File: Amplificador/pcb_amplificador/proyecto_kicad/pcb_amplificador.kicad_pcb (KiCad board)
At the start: 2 copper layers, 149.9 x 88.9 mm, 140 parts, among them CON1 SJ-3523-SMT-TR, J1 Screw_Terminal_01x02, J2 Screw_Terminal_01x02, J3 Screw_Terminal_01x02, J4 Screw_Terminal_01x02, J5 Conn_01x03_Male, J6 Screw_Terminal_01x02, J7 Screw_Terminal_01x02, K1 FINDER-40.11-2016, M1 FDS9934C, M2 FDS9934C, Q1 BC860, Q10 BD139, Q11 BD140, Q12 BD139, Q13 2SA1943-O_Q_, Q14 2SC5200-O_Q, Q15 2SA1943-O_Q_, Q16 2SC5200-O_Q, Q17 2SAR514P5, Q18 BC860, Q19 BC860, Q2 BC860, Q20 2SAR514P5, Q21 2SCR514P5, Q22 2SCR514P5, Q23 2SCR514P5, Q24 2SAR514P5, Q25 2SCR514P5, Q26 BC817, Q27 BC817, Q28 BC807, Q29 BS170, Q3 BC850, Q4 BC850, Q5 BC860, Q6 BC860, Q7 BC850, Q8 2SCR514P5, Q9 2SCR514P5

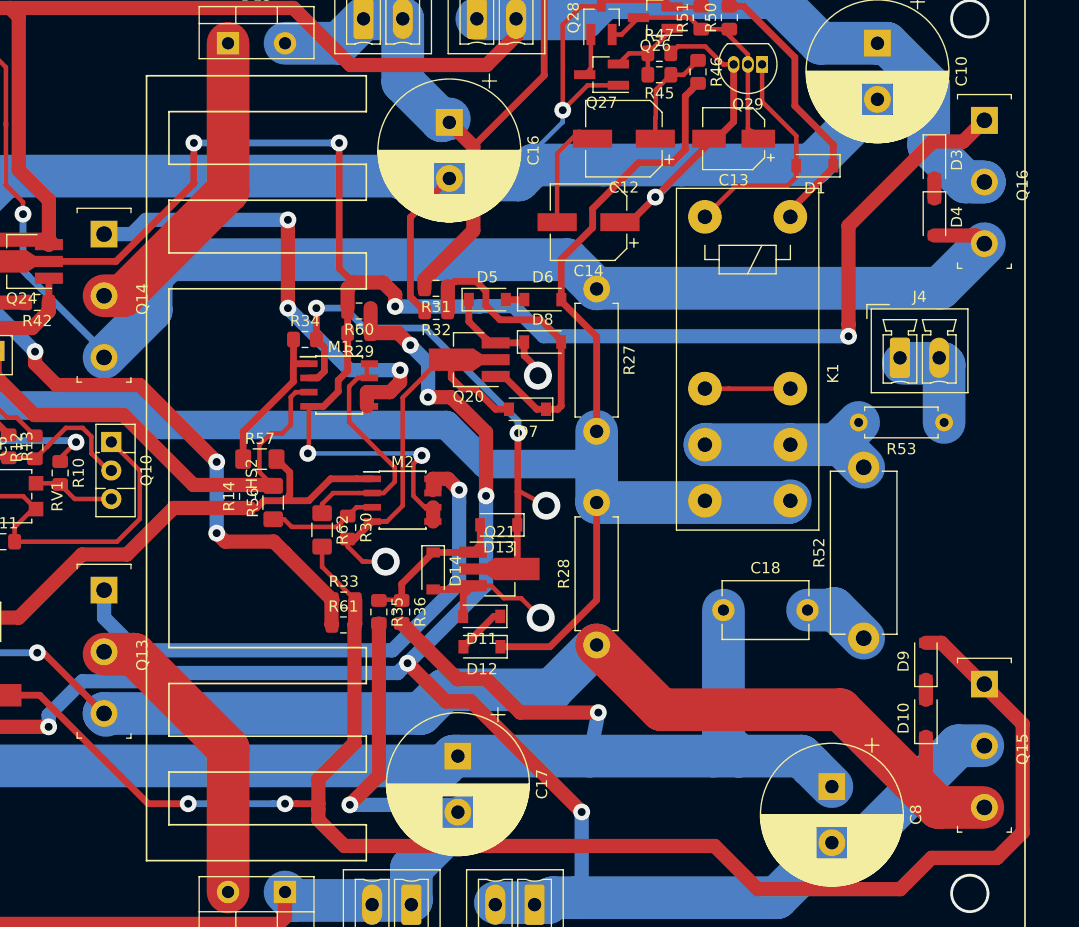
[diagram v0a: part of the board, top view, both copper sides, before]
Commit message: Agregado de las mediciones finales y algunos cambios menores
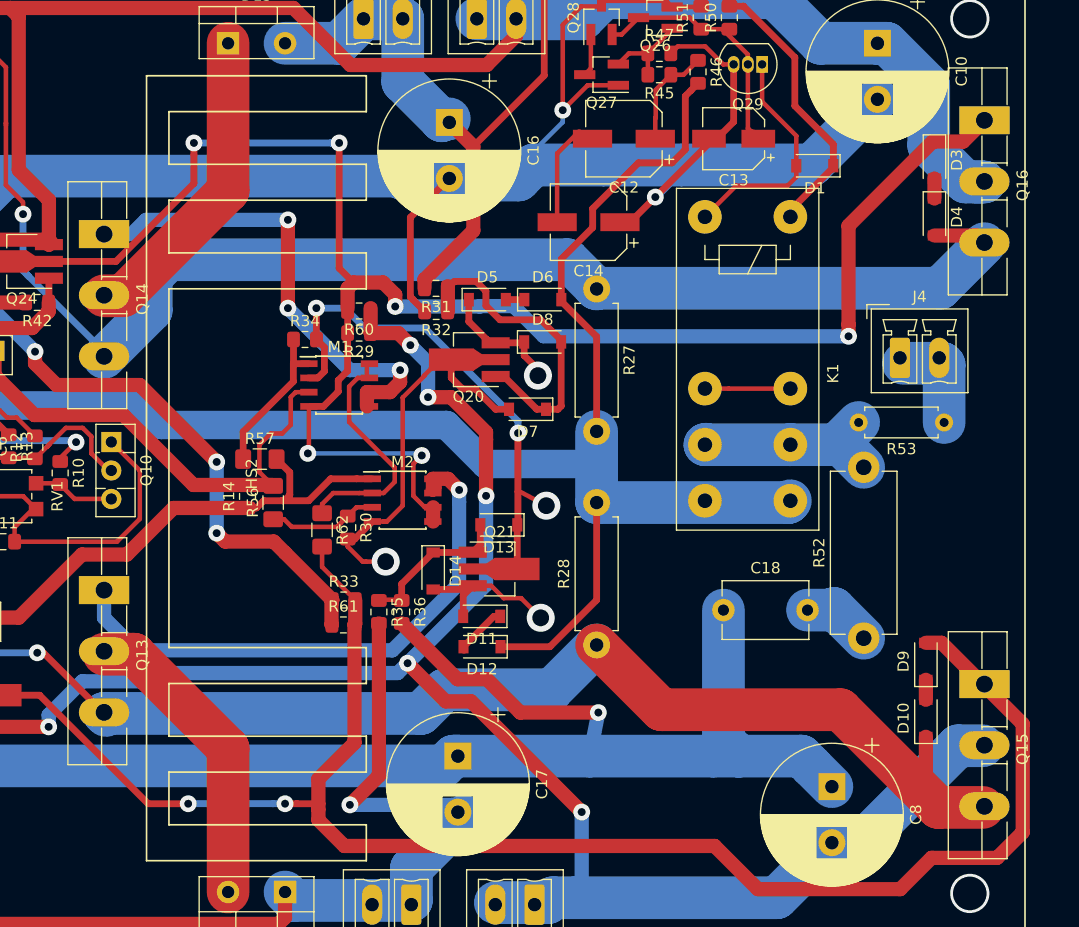
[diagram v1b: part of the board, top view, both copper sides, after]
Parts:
- Q13, Q14, Q15, Q16: footprint digikey-footprints:TO-3P-5 -> Package_TO_SOT_THT:TO-264-3_Vertical
